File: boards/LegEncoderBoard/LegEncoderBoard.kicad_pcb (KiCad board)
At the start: 2 copper layers, 34 x 42.5 mm, 5 parts, among them J1 S6B-PH-SM4-TB

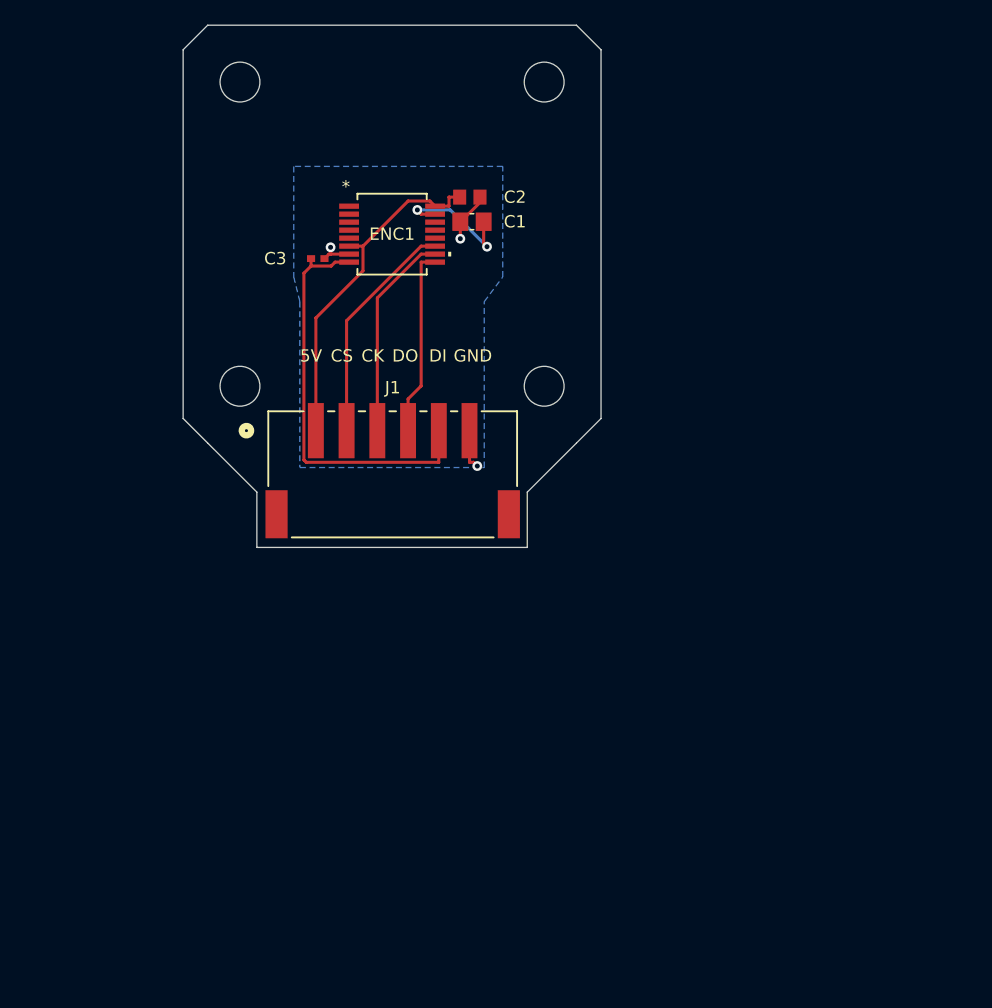
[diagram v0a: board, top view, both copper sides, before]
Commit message: Pre-final leg encoder board
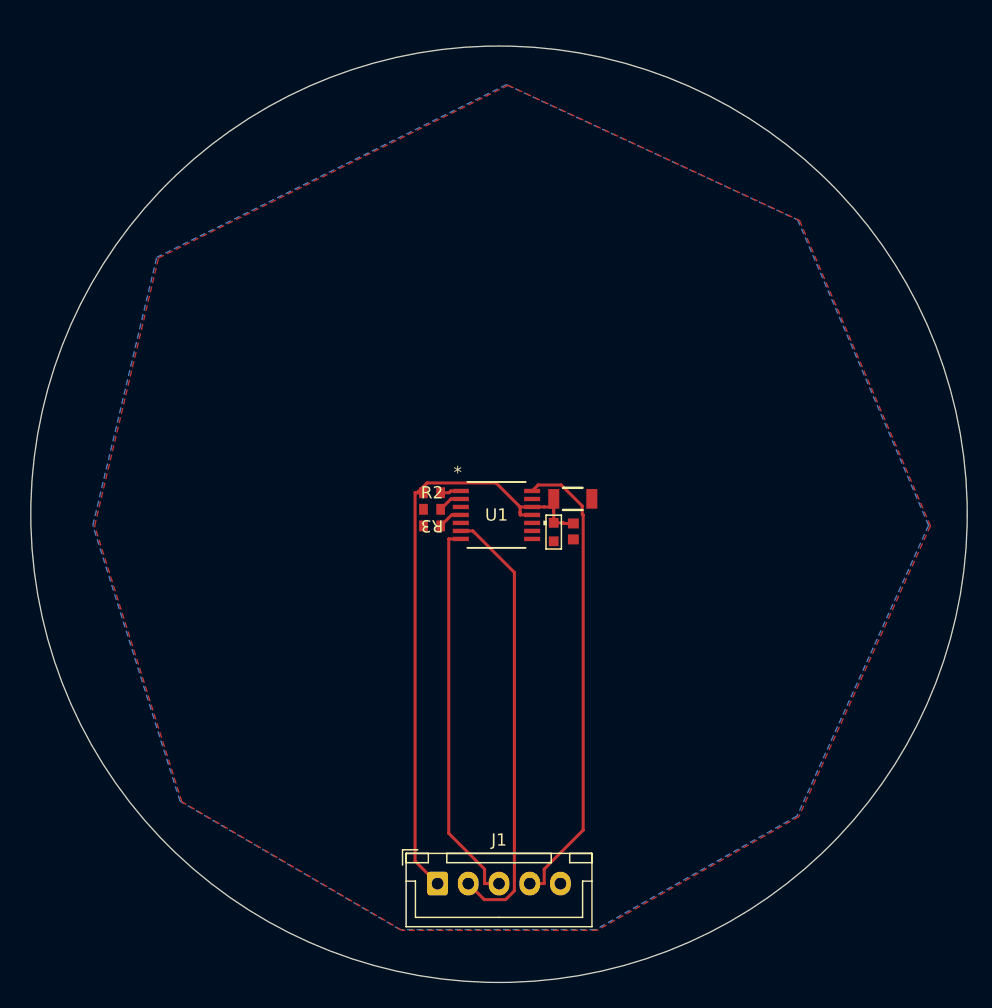
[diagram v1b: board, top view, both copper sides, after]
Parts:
- removed ENC1: AS5045-ASST, AS5045:SSOP16_AS5040-ASST_AMS
- added R1: 4.7K, Resistor4.7K:CR0603-FX-4701ELF, F.Cu at (141.8, 104.4)
- added R2: 4.7K, Resistor4.7K:CR0603-FX-4701ELF, F.Cu at (141.8, 103.0)
- added R3: 4.7K, Resistor4.7K:CR0603-FX-4701ELF, F.Cu at (141.8, 105.8)
- added U1: AS5047P-ATST, AS5047P-ASST:AS5047P-ASST, F.Cu at (147.0, 104.9)
- C1: value CC0805KKX5R7BB106 -> 100nF; footprint AS5045-3V3-REG-CAP:CAPC2012X70 -> Capacitor100nF:885342208002
- C2: value CC0805KRX7R7BB104 -> 10nF; footprint AS5045-DECOP-CAP:CC0805N_YAG -> Capacitor10nF:885012206089
- C3: value CC0402KRX7R7BB104 -> 1uF; footprint AS5045-PROG-CAP:YAG_CC0402_YAG -> Capacitor1uF:CC0603JRX7R7BB105
- J1: value S6B-PH-SM4-TB -> Conn_01x05; footprint JST-XH-6:CONN_S6B-XH-SM4-TB_JST -> Connector_JST:JST_XH_B5B-XH-A_1x05_P2.50mm_Vertical
- moved J1 33.5 mm to (142.2, 134.8)
- moved C3 30.4 mm to (153.2, 106.2), turned to 90 degrees
- moved C2 28.1 mm to (151.7, 106.2), turned to -90 degrees
- moved C1 24.0 mm to (153.2, 103.5)
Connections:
- C1 pad 1: GND -> VIN
- C1 pad 2: Net-(ENC1-VDD3V3) -> GND
- C2 pad 1: +5V -> VIN
- C3 pad 1: Net-(ENC1-PROG) -> GND
- C3 pad 2: GND -> VIN
- J1 pad 1: +5V -> VIN
- J1 pad 2: Net-(ENC1-CSN) -> A
- J1 pad 3: Net-(ENC1-CLK) -> B
- J1 pad 4: Net-(ENC1-DO) -> I
- J1 pad 5: Net-(ENC1-PROG) -> GND
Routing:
- net VIN: track 0.00 -> 50.6 mm
- net I: track 0.00 -> 38.2 mm
- net A: track 0.00 -> 36.2 mm
- net Net-(ENC1-PROG): track 33.5 -> 0.00 mm
- net B: track 0.00 -> 31.4 mm
- net +5V: track 28.0 -> 0.00 mm
- net Net-(ENC1-CSN): track 18.7 -> 0.00 mm
- net Net-(ENC1-CLK): track 17.0 -> 0.00 mm
- net Net-(ENC1-DO): track 15.3 -> 0.00 mm
- net Net-(ENC1-VDD3V3): track 10.7 -> 0.00 mm, vias 2 -> 0
- net GND: track 10.1 -> 0.00 mm, vias 3 -> 0
- net MOSI: track 0.00 -> 2.01 mm
- net SCK: track 0.00 -> 1.99 mm
- net CS: track 0.00 -> 1.70 mm
- added copper zone on F.Cu, net GND
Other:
- board size 34 x 42.5 mm -> 76.2 x 76.2 mm
- board text removed: "5V"
- board text removed: "CK"
- board text removed: "CS"
- board text removed: "DI"
- board text removed: "DO"
- board text removed: "GND"

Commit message: Leg encoder board pre-final
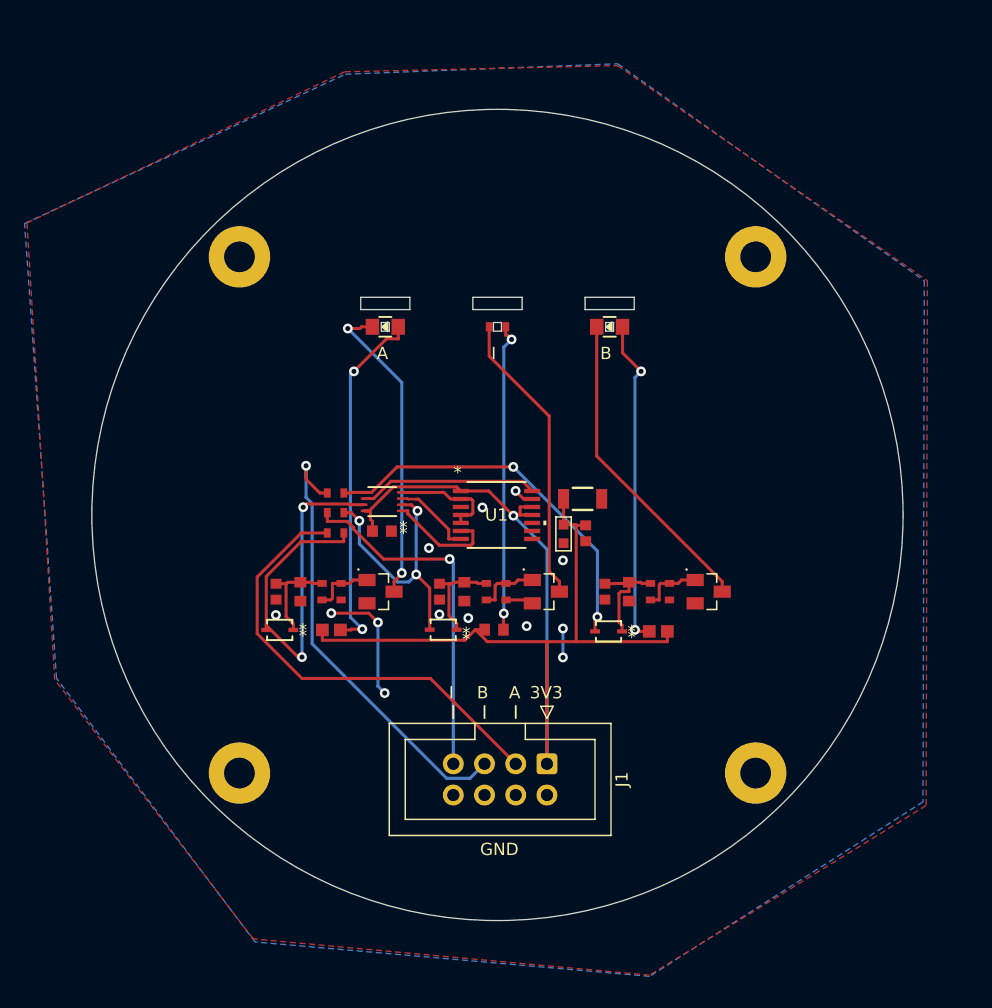
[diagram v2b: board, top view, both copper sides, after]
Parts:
- added C4: 0.1uF, Capacitor0.1uF:GRM188R71H104KA93J, F.Cu at (137.7, 106.2)
- added C5: 1uF, Capacitor1uF:CC0603JRX7R7BB105, F.Cu at (129.1, 111.1)
- added C6: 1uF, Capacitor1uF:CC0603JRX7R7BB105, F.Cu at (155.8, 111.1)
- added C7: 1uF, Capacitor1uF:CC0603JRX7R7BB105, F.Cu at (142.4, 111.1)
- added CR1: BAT54, EnvelopeDiode:BAT54WS-7-F, F.Cu at (129.4, 114.2)
- added CR2: BAT54, EnvelopeDiode:BAT54WS-7-F, F.Cu at (156.1, 114.3)
- added CR3: BAT54, EnvelopeDiode:BAT54WS-7-F, F.Cu at (142.7, 114.2)
- added D1: REDLED, RedLED:RC0603FR-07150RL, F.Cu at (147.1, 89.5)
- added D2: BLUELED, BlueLED:150080BS75000_Modified, F.Cu at (137.9, 89.5)
- added D3: BLUELED, BlueLED:150080BS75000_Modified, F.Cu at (156.2, 89.5)
- added H1: MountingHole, MountingHole:MountingHole_2.5mm_Pad, F.Cu at (126.1, 83.9)
- added H2: MountingHole, MountingHole:MountingHole_2.5mm_Pad, F.Cu at (168.1, 83.9)
- added H3: MountingHole, MountingHole:MountingHole_2.5mm_Pad, F.Cu at (126.1, 125.9)
- added H4: MountingHole, MountingHole:MountingHole_2.5mm_Pad, F.Cu at (168.1, 125.9)
- added Q1: MMBT3904, Transistor:MMBT3904LT1G, F.Cu at (137.6, 111.1)
- added Q2: MMBT3904, Transistor:MMBT3904LT1G, F.Cu at (164.3, 111.1)
- added Q3: MMBT3904, Transistor:MMBT3904LT1G, F.Cu at (151.0, 111.1)
- added R10: 100K, Resistor100K:CRCW0603100KFKEA, F.Cu at (144.4, 111.1)
- added R11: 47K, Resistor47K:RC0603FR-0747KL, F.Cu at (146.2, 111.1)
- added R12: 470K, Resistor470K:RC0603FR-07470KL, F.Cu at (147.8, 111.1)
- added R13: 22R, Resistor22:RC0603FR-0722RL, F.Cu at (133.9, 106.3)
- added R14: 22R, Resistor22:RC0603FR-0722RL, F.Cu at (133.9, 103.1)
- added R15: 22R, Resistor22:RC0603FR-0722RL, F.Cu at (133.9, 104.7)
- added R4: 1K, Resistor1K:RCG06031K00FKEA, F.Cu at (146.8, 114.2)
- added R5: 100K, Resistor100K:CRCW0603100KFKEA, F.Cu at (157.8, 111.1)
- added R6: 150R, Resistor150:RESC1607X60N, F.Cu at (133.6, 114.2)
- added R7: 47K, Resistor47K:RC0603FR-0747KL, F.Cu at (159.5, 111.1)
- added R8: 470K, Resistor470K:RC0603FR-07470KL, F.Cu at (161.1, 111.1)
- added R9: 150R, Resistor150:RESC1607X60N, F.Cu at (160.2, 114.3)
- added U2: SN74LVC3G17DCUR, SchmittBuffer:SN74LVC3G17DCUR, F.Cu at (137.7, 103.8)
- J1: footprint Connector_JST:JST_XH_B5B-XH-A_1x05_P2.50mm_Vertical -> Connector_IDC:IDC-Header_2x04_P2.54mm_Vertical
- R1: value 4.7K -> 100K; footprint Resistor4.7K:CR0603-FX-4701ELF -> Resistor100K:CRCW0603100KFKEA
- R2: value 4.7K -> 47K; footprint Resistor4.7K:CR0603-FX-4701ELF -> Resistor47K:RC0603FR-0747KL
- R3: value 4.7K -> 470K; footprint Resistor4.7K:CR0603-FX-4701ELF -> Resistor470K:RC0603FR-07470KL
- moved J1 13.2 mm to (151.1, 125.1), turned to -90 degrees
- moved R1 12.6 mm to (131.0, 111.1), turned to -90 degrees
- moved R2 12.0 mm to (132.8, 111.1), turned to -90 degrees
- moved R3 9.13 mm to (134.4, 111.1), turned to -90 degrees
- moved C3 1.01 mm to (154.2, 106.3)
- moved C2 0.81 mm to (152.4, 106.4)
- moved C1 0.80 mm to (154.0, 103.5)
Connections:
- J1 pad 2: A -> GND
- J1 pad 3: B -> /A_OUT
- J1 pad 4: I -> GND
- J1 pad 5: GND -> /B_OUT
- R1 pad 1: SCK -> /A_ENV
- R2 pad 1: VIN -> /A_ENV
- R2 pad 2: CS -> /A_BASE
- R3 pad 1: MOSI -> /A_BASE
- U1 pad 1: CS -> VIN
- U1 pad 2: SCK -> GND
- U1 pad 3: MISO -> unconnected-(U1-MISO-Pad3)
- U1 pad 4: MOSI -> GND
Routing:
- net VIN: track 50.6 -> 95.2 mm, vias 0 -> 1
- net /A_OUT: track 0.00 -> 37.2 mm
- net /B_OUT: track 0.00 -> 37.0 mm, vias 0 -> 1
- net A_BUF: track 0.00 -> 33.9 mm, vias 0 -> 2
- net B_BUF: track 0.00 -> 31.0 mm, vias 0 -> 2
- net /A_LED_ANODE: track 0.00 -> 29.0 mm, vias 0 -> 2
- net /I_OUT: track 0.00 -> 28.8 mm, vias 0 -> 1
- net A: track 36.2 -> 9.26 mm
- net /B_LED_ANODE: track 0.00 -> 26.7 mm, vias 0 -> 2
- net /B_LED_CATHODE: track 0.00 -> 25.8 mm
- net /A_LED_CATHODE: track 0.00 -> 25.5 mm, vias 0 -> 2
- net /I_LED_ANODE: track 0.00 -> 25.2 mm, vias 0 -> 2
- net GND: track 0.00 -> 25.2 mm, vias 0 -> 13
- net B: track 31.4 -> 6.73 mm
- net /I_LED_CATHODE: track 0.00 -> 23.9 mm
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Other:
- board size 76.2 x 76.2 mm -> 66 x 66 mm
- board text added: "3V3"
- board text added: "A"
- board text added: "B"
- board text added: "GND"
- board text added: "I"
